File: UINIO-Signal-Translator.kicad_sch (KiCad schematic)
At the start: 3 parts, among them J1 Conn_01x08_Pin, J3 Conn_01x08_Pin, U1 TXS0108EPW

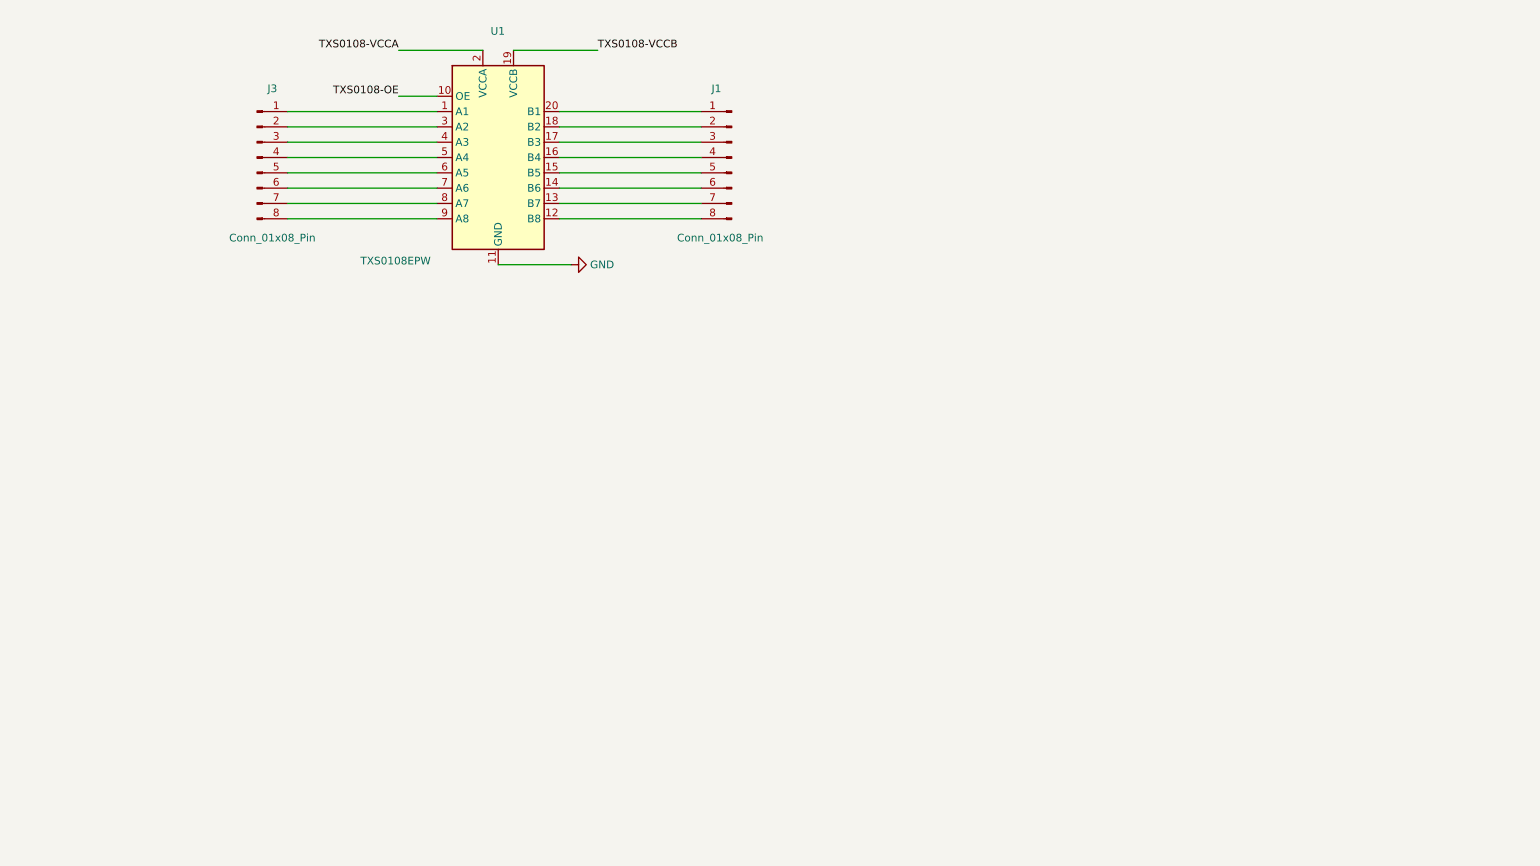
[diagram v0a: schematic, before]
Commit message: Release UINIO-Signal-Translator version 1.0.0.
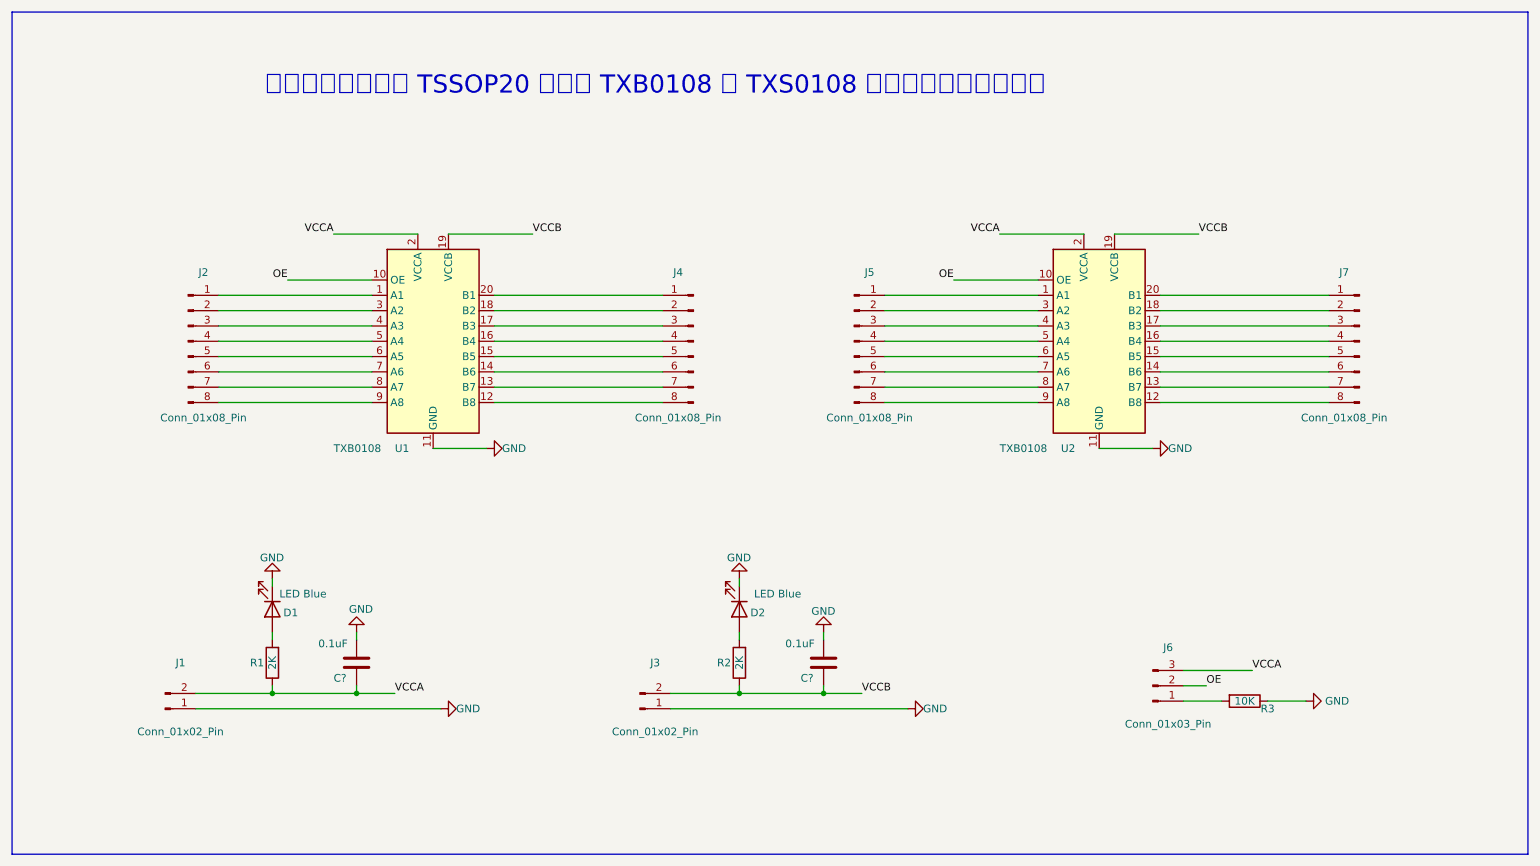
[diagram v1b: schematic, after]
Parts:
- removed J1, J3: Conn_01x08_Pin, symbol Connector:Conn_01x08_Pin
- added C? (x2): 0.1uF, Capacitor_SMD:C_0603_1608Metric, symbol Device:C
- added D1, D2: LED Blue, LED_SMD:LED_0603_1608Metric, symbol Device:LED
- added J1, J3: Conn_01x02_Pin, Connector_PinHeader_2.54mm:PinHeader_1x02_P2.54mm_Vertical, symbol Connector:Conn_01x02_Pin
- added J2, J4, J5, J7: Conn_01x08_Pin, Connector_PinHeader_2.54mm:PinHeader_1x08_P2.54mm_Vertical, symbol Connector:Conn_01x08_Pin
- added J6: Conn_01x03_Pin, Connector_PinHeader_2.54mm:PinHeader_1x03_P2.54mm_Vertical, symbol Connector:Conn_01x03_Pin
- added R1, R2: 2K, Resistor_SMD:R_0603_1608Metric, symbol Device:R
- added R3: 10K, Resistor_SMD:R_0603_1608Metric, symbol Device:R
- added U2: TXB0108, Package_SO:TSSOP-20_4.4x6.5mm_P0.65mm, symbol Logic_LevelTranslator:TXS0108EPW
- U1: value TXS0108EPW -> TXB0108
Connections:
- net GND: now also C?.1, C?.1, D1.1 (K), D2.1 (K), J1.1 (Pin_1), J3.1 (Pin_1), R3.1, U2.11 (GND)
- net at U1.1 (A1): now also J2.1 (Pin_1)
- net at U1.3 (A2): now also J2.2 (Pin_2)
- net at U1.4 (A3): now also J2.3 (Pin_3)
- net at U1.5 (A4): now also J2.4 (Pin_4)
- net at U1.6 (A5): now also J2.5 (Pin_5)
- net at U1.7 (A6): now also J2.6 (Pin_6)
- net at U1.8 (A7): now also J2.7 (Pin_7)
- net at U1.9 (A8): now also J2.8 (Pin_8)
- net at U1.12 (B8): now also J4.8 (Pin_8)
- net at U1.13 (B7): now also J4.7 (Pin_7)
- net at U1.14 (B6): now also J4.6 (Pin_6)
- net at U1.15 (B5): now also J4.5 (Pin_5)
- net at U1.16 (B4): now also J4.4 (Pin_4)
- net at U1.17 (B3): now also J4.3 (Pin_3)
- net at U1.18 (B2): now also J4.2 (Pin_2)
- net at U1.20 (B1): now also J4.1 (Pin_1)
- net TXS0108-OE renamed OE
- net OE: now also J6.2 (Pin_2), U2.10 (OE)
- net TXS0108-VCCA renamed VCCA
- net VCCA: now also C?.2, J1.2 (Pin_2), J6.3 (Pin_3), R1.1, U2.2 (VCCA)
- net TXS0108-VCCB renamed VCCB
- net VCCB: now also C?.2, J3.2 (Pin_2), R2.1, U2.19 (VCCB)
- new net: J5.1 (Pin_1), U2.1 (A1)
- new net: J7.8 (Pin_8), U2.12 (B8)
- new net: J7.7 (Pin_7), U2.13 (B7)
- new net: J7.6 (Pin_6), U2.14 (B6)
- new net: J7.5 (Pin_5), U2.15 (B5)
- new net: J7.4 (Pin_4), U2.16 (B4)
- new net: J7.3 (Pin_3), U2.17 (B3)
- new net: J7.2 (Pin_2), U2.18 (B2)
- new net: J7.1 (Pin_1), U2.20 (B1)
- new net: J5.2 (Pin_2), U2.3 (A2)
- new net: J5.3 (Pin_3), U2.4 (A3)
- new net: J5.4 (Pin_4), U2.5 (A4)
- new net: J5.5 (Pin_5), U2.6 (A5)
- new net: J5.6 (Pin_6), U2.7 (A6)
- new net: J5.7 (Pin_7), U2.8 (A7)
- new net: J5.8 (Pin_8), U2.9 (A8)
- new net: D1.2 (A), R1.2
- new net: D2.2 (A), R2.2
- new net: J6.1 (Pin_1), R3.2
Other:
- note added: "同时兼容德州仪器 TSSOP20 封装的 TXB0108 与 TXS0108 两款逻辑电平转换芯片"
- moved on the sheet: U1
